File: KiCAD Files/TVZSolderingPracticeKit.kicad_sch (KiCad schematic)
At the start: 44 parts, among them J1 Barrel Jack, J2 Conn_01x05_Pin, J3 Conn_01x05_Socket, J4 Conn_01x03_Pin, J5 Conn_01x03_Pin, SW1 SW_Push, SW10 POWER, SW11 C/D, SW2 SW_Push, SW3 SW_Push, SW4 SW_Push, SW5 SW_Push, SW6 SW_Push, SW7 SW_Push, SW8 SW_Push, U1 NE555P

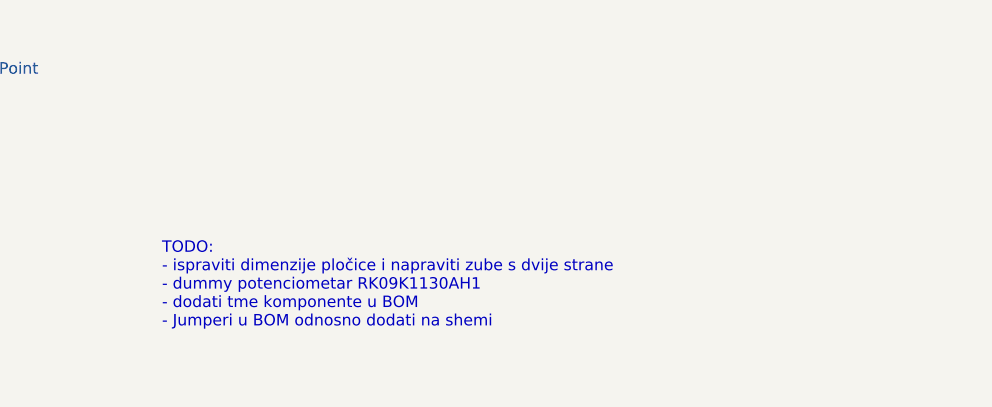
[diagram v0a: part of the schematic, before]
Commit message: update
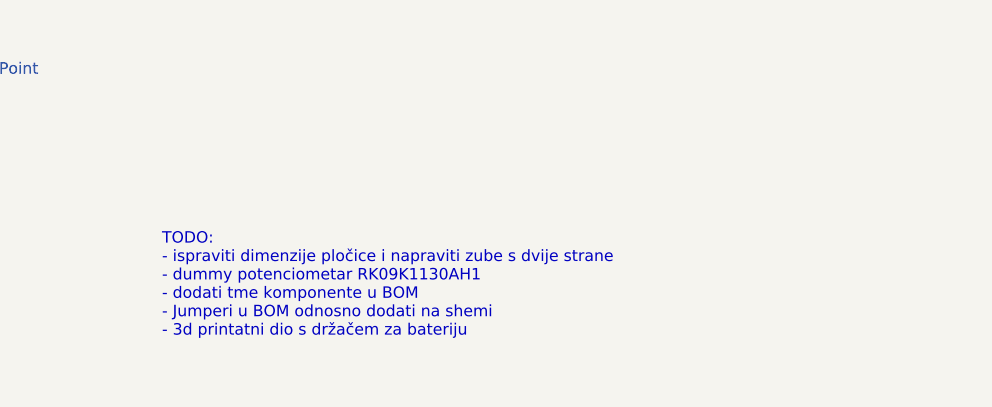
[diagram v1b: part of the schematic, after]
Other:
- note added: "TODO: - ispraviti dimenzije pločice i napraviti zube s dvije strane - dummy potenciometar RK09K1130AH1 - dodati tme komponente u BOM - Jumperi u BOM odnosno dodati na shemi - 3d printatni dio s držačem za bateriju"
- note removed: "TODO: - ispraviti dimenzije pločice i napraviti zube s dvije strane - dummy potenciometar RK09K1130AH1 - dodati tme komponente u BOM - Jumperi u BOM odnosno dodati na shemi"
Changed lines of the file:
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@@
 	(generator_version "9.0")
 	(paper "A4")
-	(text "TODO:\n- ispraviti dimenzije pločice i napraviti zube s dvije strane\n- dummy potenciometar RK09K1130AH1\n- dodati tme komponente u BOM\n- Jumperi u BOM odnosno dodati na shemi\n"
+	(text "TODO:\n- ispraviti dimenzije pločice i napraviti zube s dvije strane\n- dummy potenciometar RK09K1130AH1\n- dodati tme komponente u BOM\n- Jumperi u BOM odnosno dodati na shemi\n- 3d printatni dio s držačem za bateriju\n"
 		(exclude_from_sim no)
 		(at 86.614 174.498 0)
